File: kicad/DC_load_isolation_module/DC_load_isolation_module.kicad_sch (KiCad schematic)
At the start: 4 parts

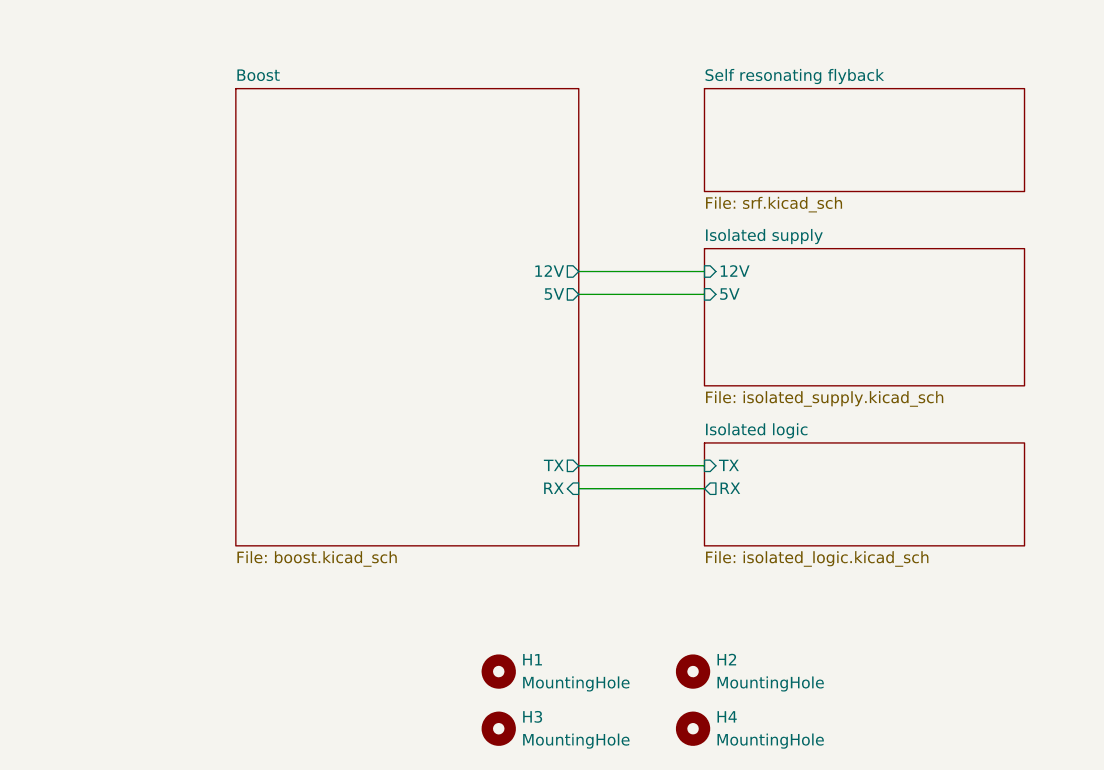
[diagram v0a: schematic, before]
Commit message: SRF layout
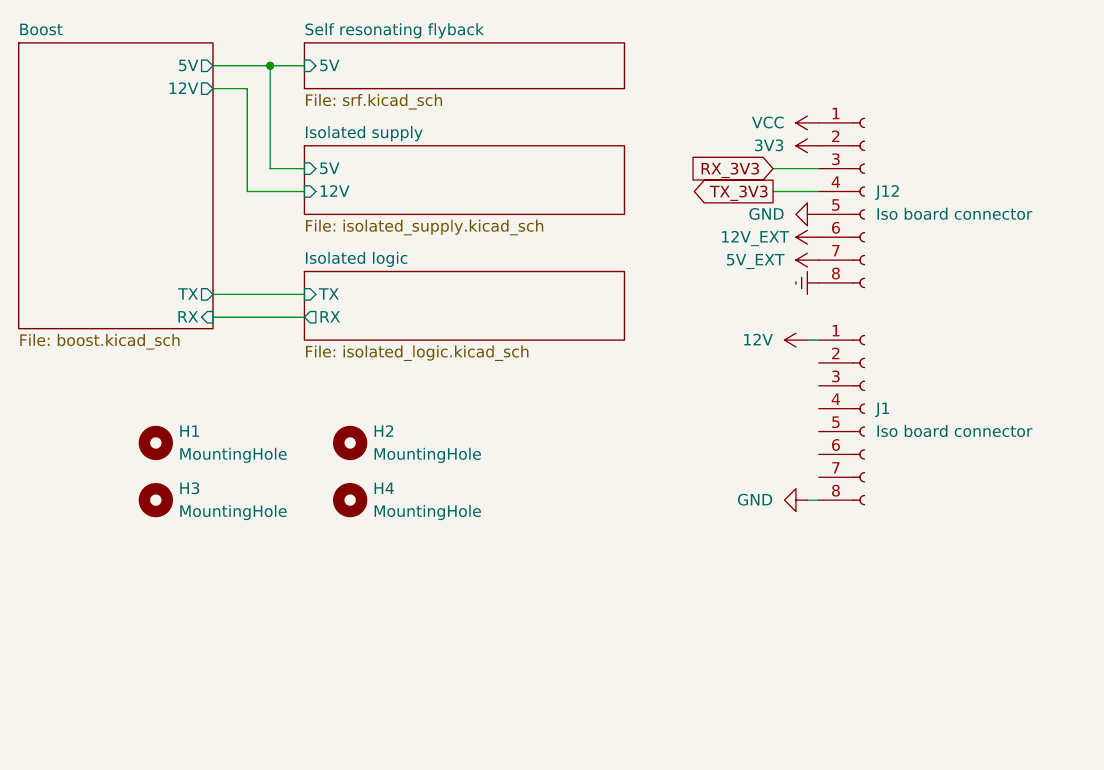
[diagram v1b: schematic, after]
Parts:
- added J1, J12: Iso board connector, Connector_PinSocket_2.54mm:PinSocket_1x08_P2.54mm_Vertical, symbol Connector:Conn_01x08_Socket
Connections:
- new net 12V: J1.1 (Pin_1)
- new net 12V_EXT: J12.6 (Pin_6)
- new net 3V3: J12.2 (Pin_2)
- new net 5V_EXT: J12.7 (Pin_7)
- new net Earth: J12.8 (Pin_8)
- new net GND: J1.8 (Pin_8), J12.5 (Pin_5)
- new net RX_3V3: J12.3 (Pin_3)
- new net TX_3V3: J12.4 (Pin_4)
- new net VCC: J12.1 (Pin_1)
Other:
- sheet Self resonating flyback ports: added 5V; removed none
- moved on the sheet: H1, H2, H3, H4
